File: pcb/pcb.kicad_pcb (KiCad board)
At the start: 2 copper layers, 149.6 x 66.4 mm, 34 parts, among them J1 Ribbon Cable Header, J2 Ribbon Cable Header, J3 UPDI, SW1 MX Grey w/ LED, SW2 MX Grey w/ LED, SW3 1241.1100.7095, SW4 SW_SPST, U1 Display Driver, U2 Display Driver, U3 MCU, U4 OR, 2 Channels, U5 Voltage Regulator, Y1 32.768 kHz

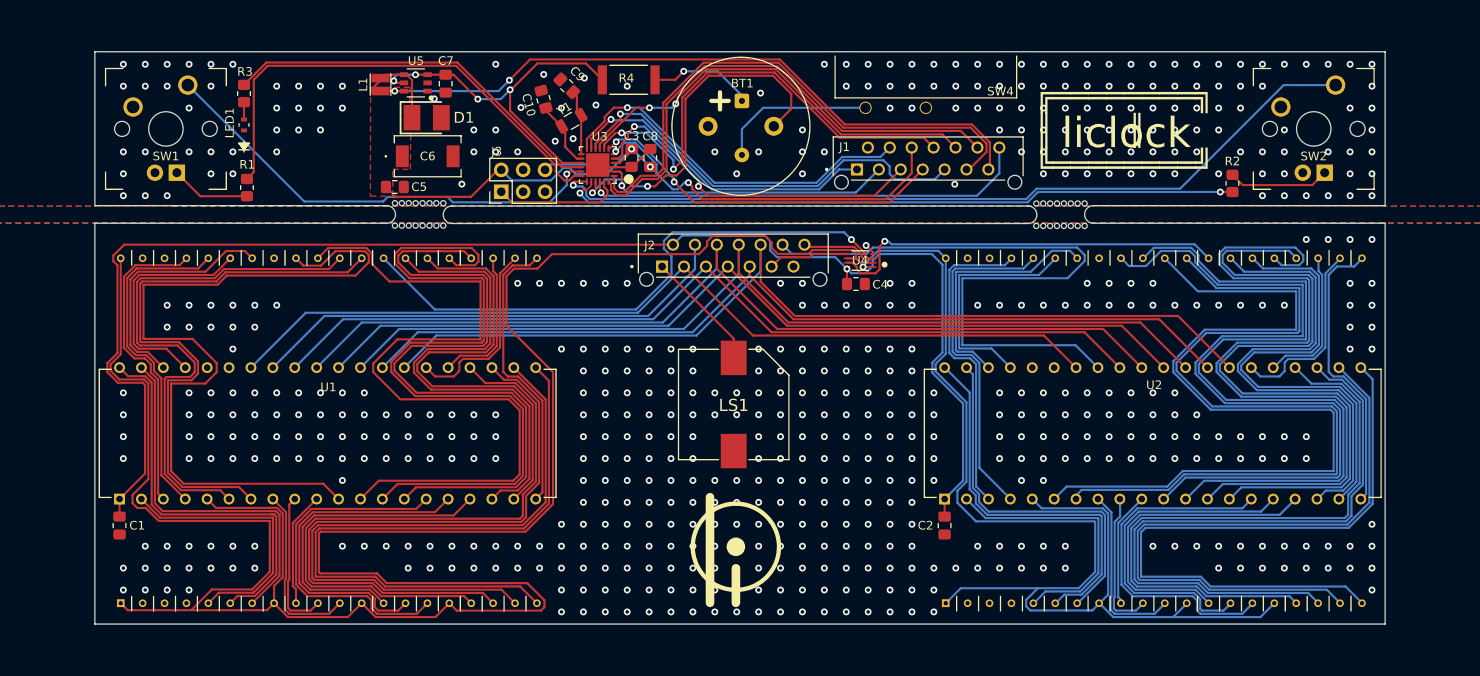
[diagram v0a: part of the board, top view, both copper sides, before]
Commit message: Redo pcb layout
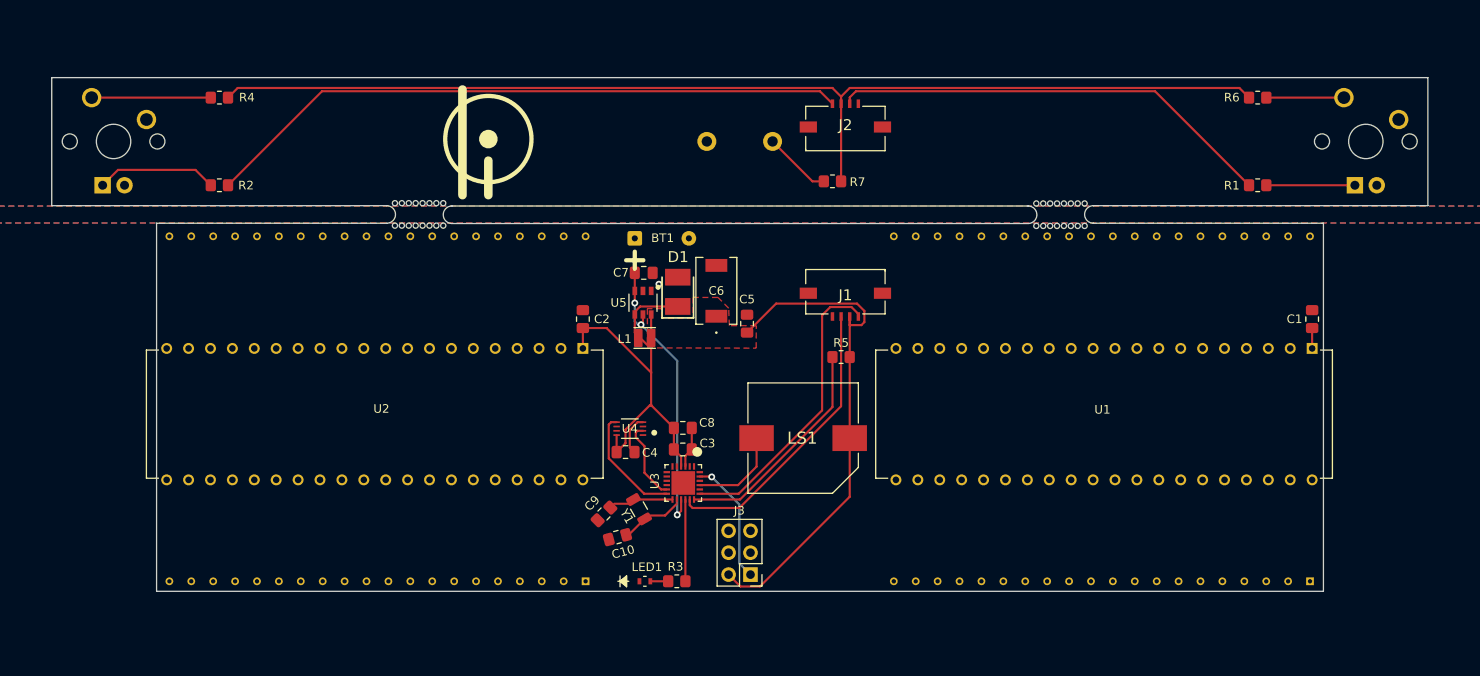
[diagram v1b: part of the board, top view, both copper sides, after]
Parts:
- removed SW4: SW_SPST, chess_clock:CWSA11AAN1H
- added R5: 2.7kΩ, Resistor_SMD:R_0805_2012Metric_Pad1.20x1.40mm_HandSolder, F.Cu at (161.2, 109.5)
- added R6: 27kΩ, Resistor_SMD:R_0805_2012Metric_Pad1.20x1.40mm_HandSolder, F.Cu at (209.5, 79.4)
- added R7: 12kΩ, Resistor_SMD:R_0805_2012Metric_Pad1.20x1.40mm_HandSolder, F.Cu at (160.2, 89.1)
- J1, J2: value Ribbon Cable Header -> Conn_01x04; footprint chess_clock:903250014 -> chess_clock:2005290040
- LCD1, LCD2, SW1, SW2, SW3: moved to B.Cu
- R4: value 50Ω -> 2.7kΩ; footprint chess_clock:352151RFT -> Resistor_SMD:R_0805_2012Metric_Pad1.20x1.40mm_HandSolder
- Y1: value 32.768 kHz -> 32kHz
- moved C1 140.3 mm to (215.8, 105.1), turned to -90 degrees
- moved U1 139.4 mm to (215.8, 108.5), turned to -90 degrees
- moved SW2 139.2 mm to (76.8, 84.5), turned to 180 degrees
- moved SW1 139.1 mm to (222.0, 84.5), turned to 180 degrees
- moved R2 117.5 mm to (89.1, 89.6), turned to 0 degrees
- moved R1 117.2 mm to (209.5, 89.6), turned to 180 degrees
- moved LCD2 90.1 mm to (107.4, 115.5)
- moved LCD1 89.7 mm to (191.4, 115.5)
- moved R3 75.6 mm to (142.2, 135.5), turned to 0 degrees
- moved LED1 70.4 mm to (138.5, 135.5), turned to 0 degrees
- moved J3 53.0 mm to (150.7, 134.7), turned to 180 degrees
- moved C10 51.5 mm to (135.3, 130.4), turned to 15 degrees
- moved C9 49.8 mm to (133.7, 127.7), turned to 45 degrees
- moved C2 48.3 mm to (131.3, 105.1), turned to -90 degrees
- moved R4 47.5 mm to (89.1, 79.4)
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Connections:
- net /LED1_ENABLE renamed /BAT_LOW_LED
- net UDPI renamed UPDI
- BT1 pad 1: Net-(BT1-+) -> VBAT
- BT1 pad 2: Net-(BT1--) -> GND
- C1 pad 1: VSS -> GND
- C1 pad 2: VDD -> VCC
- C2 pad 1: VSS -> GND
- C2 pad 2: VDD -> VCC
- C4 pad 1: VDD -> VCC
- C4 pad 2: VSS -> GND
- C7 pad 1: VBAT_PROT -> VBAT
- J1 pad 1: LCD_COL_2 -> /SW2_LED
- J1 pad 2: GND -> VCC
- J1 pad 3: LCD_LATCH_2 -> /SW1_LED
- J1 pad 4: LCD_COL_1 -> GND
- J1 pad 5: LCD_DATA0 -> GND
- J1 pad 6: LCD_DATA1 -> GND
- J2 pad 1: /BUZZ -> Net-(J2-Pad1)
- J2 pad 2: VDD -> Net-(J2-Pad2)
- J2 pad 3: WRITE -> Net-(J2-Pad3)
- J2 pad 4: LATCH_1 -> GND1
- J2 pad 5: DIGIT2 -> GND1
- J2 pad 6: DIGIT1 -> GND1
- LS1 pad 1: /BUZZ -> VCC
- LS1 pad 2: VSS -> /BUZZ
- R1 pad 1: /SW1_LED_ENABLE -> Net-(SW1-A)
- R1 pad 2: Net-(SW1-A) -> Net-(J2-Pad3)
- R2 pad 1: /SW2_LED_ENABLE -> Net-(SW2-A)
- R2 pad 2: Net-(SW2-A) -> Net-(J2-Pad1)
- R4 pad 1: Net-(BT1-+) -> Net-(J2-Pad2)
- R4 pad 2: VBAT_PROT -> Net-(R4-Pad2)
- SW1 pad 1: GND -> GND1
- SW1 pad 2: /~{SW1_ACTIVE} -> Net-(R6-Pad1)
- SW1 pad 3: GND -> GND1
- SW2 pad 1: GND -> GND1
- SW2 pad 2: /~{SW2_ACTIVE} -> Net-(R4-Pad2)
- SW2 pad 3: GND -> GND1
- SW3 pad 1: GND -> Net-(R7-Pad1)
- SW3 pad 2: /~{SW3_ACTIVE} -> GND1
- U1 pad 1: VDD -> VCC
- U1 pad 34: WRITE -> LCD_WRITE
- U1 pad 35: VSS -> GND
- U2 pad 1: VDD -> VCC
- U2 pad 34: WRITE -> LCD_WRITE
- U2 pad 35: VSS -> GND
- U2 pad 36: VSS -> GND
- U3 pad 1: LCD_LATCH_1 -> LATCH_1
- U3 pad 10: LCD_DIGIT1 -> DIGIT1
- U3 pad 11: LCD_COL_2 -> COL_2
- U3 pad 12: LCD_COL_1 -> COL_1
- U3 pad 15: VBAT_PROT -> VBAT
- U3 pad 17: /~{SW1_ACTIVE} -> /SW1_LED
- U3 pad 18: /SW1_LED_ENABLE -> /SW_READ
- U3 pad 19: /~{SW2_ACTIVE} -> /SW2_LED
- U3 pad 2: LCD_LATCH_2 -> LATCH_2
- U3 pad 20: /SW2_LED_ENABLE -> unconnected-(U3-PC3-Pad20)
- U3 pad 21: /~{SW3_ACTIVE} -> /BUZZ
- U3 pad 22: LCD_BUZZ -> unconnected-(U3-PC5-Pad22)
- U3 pad 5: LCD_DATA0 -> DATA0
- U3 pad 6: LCD_DATA1 -> DATA1
- U3 pad 7: LCD_DATA2 -> DATA2
- U3 pad 8: LCD_DATA3 -> DATA3
- U3 pad 9: LCD_DIGIT2 -> DIGIT2
- U4 pad 4: VSS -> GND
- U4 pad 8: VDD -> VCC
- U5 pad 3: VBAT_PROT -> VBAT
- U5 pad 5: VBAT_PROT -> VBAT
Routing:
- net BP: track 417.5 -> 0.00 mm, vias 1 -> 0
- net VDD: track 171.1 -> 0.00 mm, vias 1 -> 0
- net Net-(J2-Pad2): track 0.00 -> 130.0 mm
- net DIGIT1: track 113.6 -> 0.00 mm
- net DATA0: track 112.4 -> 0.00 mm
- net DATA2: track 111.4 -> 0.00 mm
- net DATA1: track 106.9 -> 0.00 mm
- net DATA3: track 105.6 -> 0.00 mm
- net DIGIT2: track 105.4 -> 0.00 mm
- net WRITE: track 105.4 -> 0.00 mm
- net /LCD2.A2: track 99.4 -> 0.00 mm
- net /~{SW2_ACTIVE}: track 96.9 -> 0.00 mm, vias 1 -> 0
- net /LCD2.B2: track 95.6 -> 0.00 mm
- net /LCD2.G2: track 92.7 -> 0.00 mm
- net /LCD1.G2: track 91.4 -> 0.00 mm
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- added copper zone on B.Cu, net GND1
- added copper zone on F.Cu, net GND1
- removed copper zone on B.Cu, net VSS
- removed copper zone on F.Cu, net VSS
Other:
- board size 149.6 x 66.4 mm -> 159.6 x 59.6 mm
- board text added: "0.3.0"
- board text removed: "0.2.0"
